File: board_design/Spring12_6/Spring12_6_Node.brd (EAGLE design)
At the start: 100 x 80 mm, 40 parts, among them IC1 L78S05CV, Q1 20MHz, X1 1751248

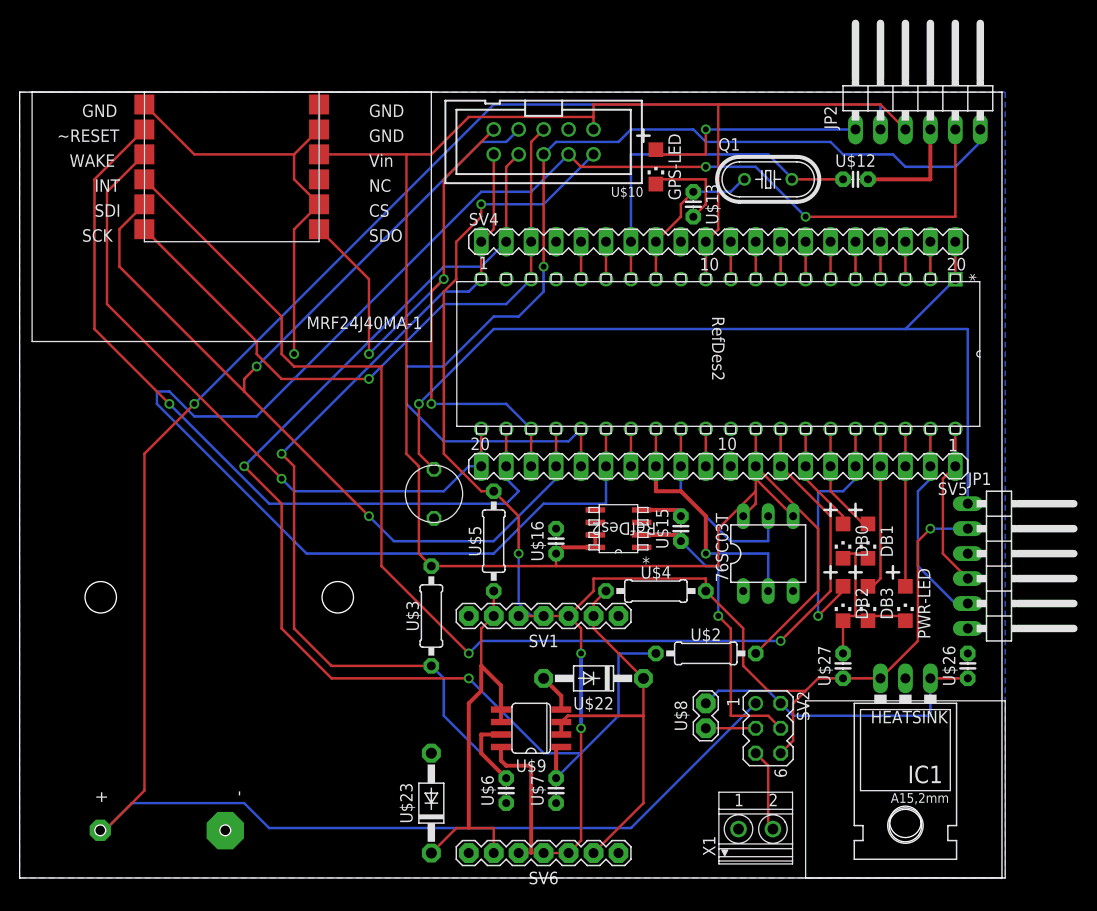
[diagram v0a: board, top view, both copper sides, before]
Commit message: PCB V2
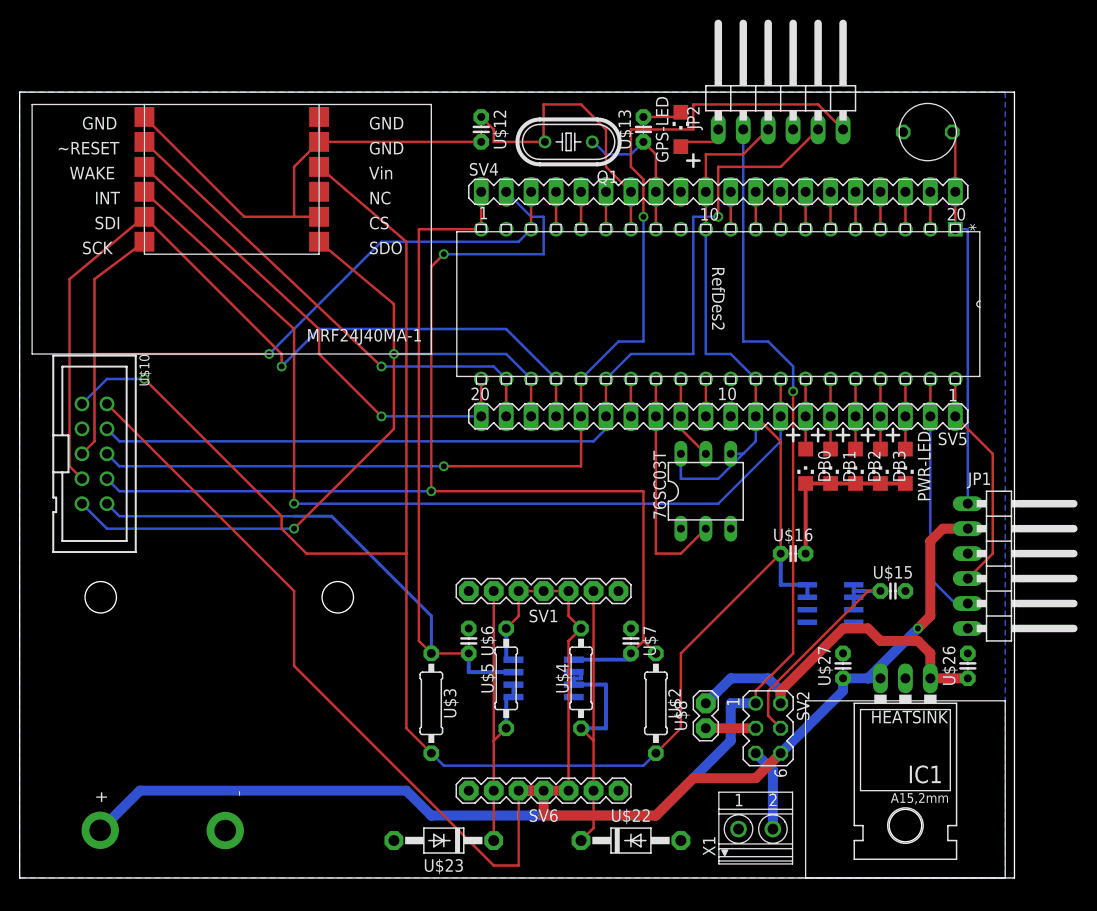
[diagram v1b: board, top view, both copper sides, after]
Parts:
- moved U$25 60.7 mm to (91.4, 74.9), turned to 270 degrees
- moved U$10 55.7 mm to (7.62, 43.2), turned to 270 degrees
- moved U$12 38.4 mm to (47.0, 76.2), turned to 270 degrees
- moved U$16 24.2 mm to (78.7, 33.0), turned to 0 degrees
- moved U$14 22.9 mm to (82.5, 27.9), flipped to the bottom, turned to 0 degrees
- moved U$15 22.5 mm to (88.9, 29.2), turned to 0 degrees
- moved Q1 20.7 mm to (55.9, 74.9), turned to 180 degrees
- moved U$7 17.0 mm to (62.2, 24.1), turned to 270 degrees
- moved U$22 16.9 mm to (62.2, 3.81), turned to 0 degrees
- moved U$6 15.7 mm to (45.7, 24.1), turned to 270 degrees
- moved U$5 14.0 mm to (49.5, 20.3)
- moved DB2 14.0 mm to (85.1, 41.9)
- moved DB3 14.0 mm to (87.6, 41.9)
- moved JP2 14.0 mm to (77.5, 80.0)
- moved PWR-LED 14.0 mm to (90.2, 41.9)
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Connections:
- net N$26: now also U$1.17
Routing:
- net UART-RX: track 167.9 -> 100.2 mm, vias 2 -> 1
- net BATTERY: track 206.7 -> 140.0 mm
- net PIC-RESET: track 95.1 -> 39.8 mm, vias 1 -> 0
- net MRF-RESET: track 80.4 -> 50.3 mm
- net MRF-INT: track 125.2 -> 97.0 mm, vias 2 -> 1
- net VSS: track 96.7 -> 71.8 mm, vias 1 -> 0
- net SPI-MOSI: track 110.9 -> 87.2 mm, vias 2 -> 1
- net 3V3: track 210.4 -> 231.9 mm, vias 0 -> 1
- net DB-LED2: track 26.2 -> 7.62 mm, vias 1 -> 0
- net MRF-WAKE: track 67.7 -> 49.8 mm
- net GPS-LED: track 23.3 -> 5.56 mm, vias 1 -> 0
- net SPI-SCK: track 66.4 -> 78.2 mm
- net I2C-ADDR1: track 19.9 -> 8.67 mm
- net DB-LED3: track 17.5 -> 7.62 mm
- net SDA-BUS: track 41.7 -> 32.4 mm
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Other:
- board size 100 x 80 mm -> 101.3 x 80 mm

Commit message: pcb stuff >_>
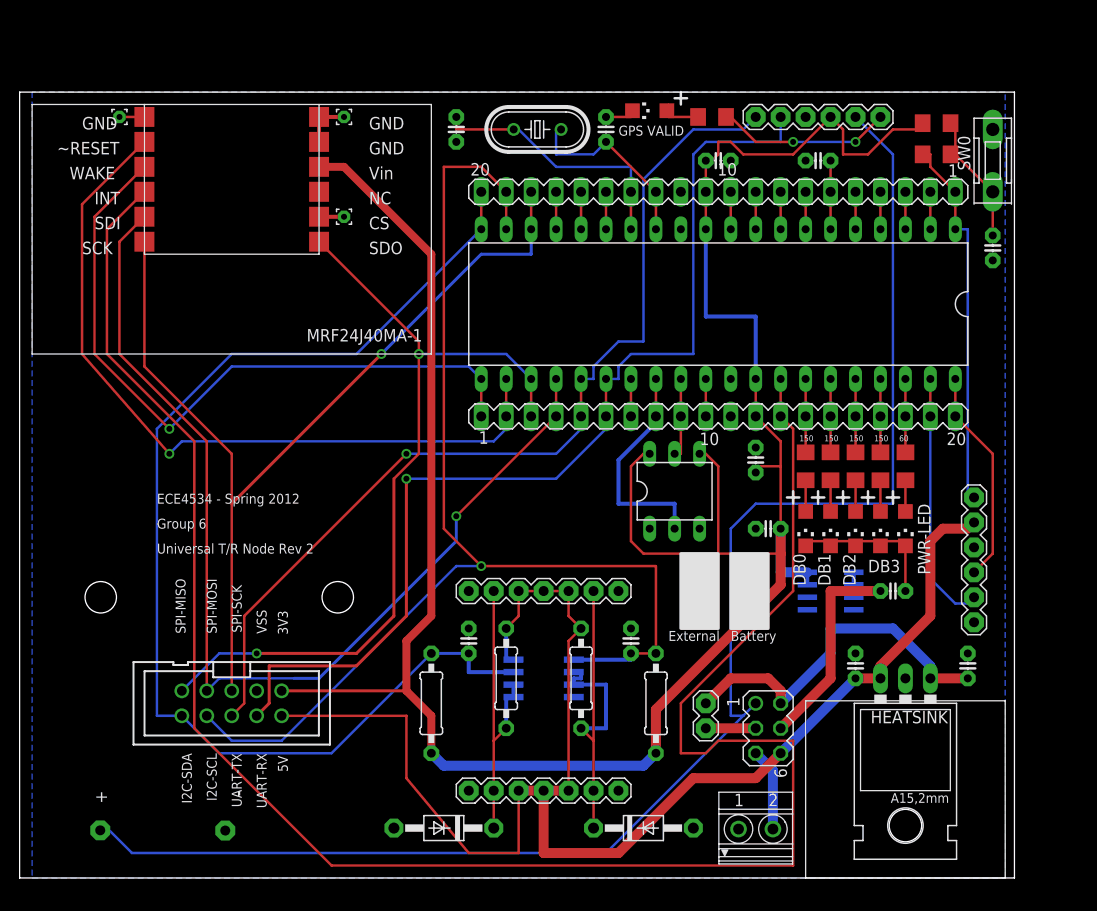
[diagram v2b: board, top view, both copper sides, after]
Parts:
- removed 76SC03T: I2C Select, ic-package:DIL06
- removed JP1: PICKIT, pinhead:1X06/90
- removed JP2: GPSR, pinhead:1X06/90
- removed U$1: PIC18F45J10-X/P, 4534_Node_Board:PDIP40_600MC
- removed U$10: DEBUG, 4534_I2C2:2510-6002
- removed U$12, U$13: 18pF, 4534_I2C2:C2.5-5
- removed U$14: MCP1725-XXXXX/SN, 4534_Node_Board:SOIC8-N_MC
- removed U$16: 10uF, 4534_I2C2:C2.5-5
- removed U$22, U$23: 1N5817P, 4534_I2C2:1N5817
- removed U$25: EVQ-11U05R, 4534_Node_Board:EVQ-11U05R
- removed U$27: 0.1uF, 4534_I2C2:C2.5-5
- added C1, C11, C8, C9: 0.1uF, 4534_I2C2:C2.5-5
- added C10, C7: 10uF, 4534_I2C2:C2.5-5
- added C2, C3: 9pF, 4534_I2C2:C2.5-5
- added D0, D1: 1N5817P, 4534_I2C2:1N5817
- added J2: DEBUG, 4534_I2C2:2510-6002
- added J3: PICKIT, 4534:MA06-1
- added J6: GPSR, 4534:MA06-1
- added PIC0: PIC18F45J10-I/P, 4534:DIL40
- added R10, R11, R8, R9: 150, 4534_I2C2:R1206
- added R4: 10k, 4534_I2C2:R1206
- added R5: 100, 4534_I2C2:R1206
- added R6, R7: 60, 4534_I2C2:R1206
- added REG0: MCP1725-XXXXX/SN, 4534_Node_Board:SOIC8-N_MC
- added SW0: SW-PB-MOM, 4534:SW-MOM-PB
- added SW1: 76SC03T, ic-package:DIL06
- added U$18, U$19, U$20: VIA, 4534_I2C2:VIA
- C4, C5: value 100pF -> 220pF
- moved DB0 6.35 mm to (80.0, 35.6)
- moved DB1 6.35 mm to (82.5, 35.6)
- moved DB2 6.35 mm to (85.1, 35.6)
- moved DB3 6.35 mm to (87.6, 35.6)
- moved PWR-LED 6.35 mm to (90.2, 35.6)
- moved GPS-LED 3.70 mm to (64.1, 78.1), turned to 90 degrees
- moved Q1 3.42 mm to (52.7, 76.2)
- turned J0 to 180 degrees
- turned J1 to 0 degrees
- renumbered IC1 to REG1, SV1 to J4, SV2 to J8, SV4 to J0, SV5 to J1, SV6 to J5, U$11 to RF0, U$15 to C6, U$17 to BATT0, U$2 to R1, U$26 to C0, U$3 to R0, U$4 to R2, U$5 to R3, U$6 to C4, U$7 to C5, U$8 to J9, U$9 to IC0, X1 to J7
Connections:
- new net N$10: DB2.A, R10.2
- new net N$11: DB3.A, R11.2
- new net N$4: GPS-LED.A, R6.2
- new net N$5: PWR-LED.A, R7.2
- new net N$6: C11.1, R4.1, R5.1, SW0.2
- new net N$7: DB0.A, R8.2
- new net N$9: DB1.A, R9.2
- net 3V3: now also C7.1, C8.1, C9.1, J0.11, J1.12, J2.1, J6.4, PIC0.11, PIC0.32, R4.2, REG0.7, REG0.8, SW1.4, SW1.6; no longer 76SC03T.4, 76SC03T.6, J0.10, J1.9, JP2.3, U$1.11, U$1.32, U$10.1, U$14.7, U$14.8, U$16.1
- net 3V3-REG: now also REG0.1, REG0.2, REG0.3; no longer U$14.1, U$14.2, U$14.3
- net 5V: now also C1.1, J2.2, J3.2; no longer JP1.2, U$10.2, U$27.1
- net BATTERY: now also J6.5; no longer JP2.2
- net DB-LED0: now also J1.14, PIC0.34, R8.1; no longer DB0.A, J1.7, U$1.34
- net DB-LED1: now also J1.15, PIC0.35, R9.1; no longer DB1.A, J1.6, U$1.35
- net DB-LED2: now also J1.16, PIC0.36, R10.1; no longer DB2.A, J1.5, U$1.36
- net DB-LED3: now also J1.17, PIC0.37, R11.1; no longer DB3.A, J1.4, U$1.37
- net GPS-LED: now also J6.6, R6.1; no longer GPS-LED.A, JP2.1
- net I2C-ADDR0: now also J1.8, PIC0.28, SW1.2; no longer 76SC03T.2, J1.13, U$1.28
- net I2C-ADDR1: now also J1.9, PIC0.29, SW1.5; no longer 76SC03T.5, J1.12, U$1.29
- net I2C-ADDR2: now also J1.10, PIC0.30; no longer J1.11, U$1.30
- net MRF-INT: now also J1.13, PIC0.33; no longer J1.8, U$1.33
- net MRF-RESET: now also J1.2, PIC0.22; no longer J1.19, U$1.22
- net MRF-WAKE: now also J1.1, PIC0.21; no longer J1.20, U$1.21
- net N$1: now also J0.8, PIC0.8; no longer J0.13, U$1.8
- net N$13: now also J0.2, PIC0.2; no longer J0.19, U$1.2
- net N$14: now also J0.3, PIC0.3; no longer J0.18, U$1.3
- net N$15: now also J0.4, PIC0.4; no longer J0.17, U$1.4
- net N$16: now also J0.5, PIC0.5; no longer J0.16, U$1.5
- net N$17: now also C10.1, J0.6, PIC0.6; no longer J0.15, U$1.6
- net N$18: now also J0.7, PIC0.7; no longer J0.14, U$1.7
- net N$2: now also J0.15, PIC0.15; no longer J0.6, U$1.15
- net N$20: now also J0.9, PIC0.9; no longer J0.12, U$1.9
- net N$21: now also J0.10, PIC0.10; no longer J0.11, U$1.10
- net N$26: now also J0.17, PIC0.17; no longer J0.4, U$1.17
- net N$3: now also J0.16, PIC0.16; no longer J0.5, U$1.16
- net N$8: now also J1.7, PIC0.27; no longer J1.14, U$1.27
- net OSC1: now also C2.1, J0.13, PIC0.13; no longer J0.8, U$1.13, U$13.1
- net OSC2: now also C3.1, J0.14, PIC0.14; no longer J0.7, U$1.14, U$12.1
- net PGC: now also J1.19, J3.5, PIC0.39; no longer J1.2, JP1.5, U$1.39
- net PGD: now also J1.20, J3.4, PIC0.40; no longer J1.1, JP1.4, U$1.40
- net PIC-RESET: now also J0.1, J3.1, PIC0.1, R5.2; no longer J0.20, JP1.1, U$1.1, U$25.P$1
- net PICKIT-AUX: now also J3.6; no longer JP1.6
- net PWR-LED: now also J1.18, PIC0.38, R7.1; no longer J1.3, PWR-LED.A, U$1.38
- net SCL-BUS: now also D1.C; no longer U$22.C
- net SCL-LOCAL: now also J0.19, J2.8, PIC0.19; no longer J0.2, U$10.8
- net SDA-BUS: now also D0.C; no longer U$23.C
- net SDA-LOCAL: now also J0.20, J2.10, PIC0.20; no longer J0.1, U$1.20, U$10.10
- net SPI-MISO: now also J1.3, J2.9, PIC0.23; no longer J1.18, U$1.23, U$10.9
- net SPI-MOSI: now also J1.4, J2.7, PIC0.24; no longer J1.17, U$1.24, U$10.7
- net SPI-SCK: now also J0.18, J2.5, PIC0.18; no longer J0.3, U$1.18, U$10.5
- net UART-RX: now also J1.6, J2.4, J6.2, PIC0.26; no longer J1.15, JP2.5, U$1.26, U$10.4
- net UART-TX: now also J1.5, J2.6, J6.1, PIC0.25; no longer J1.16, JP2.6, U$1.25, U$10.6
- net VSS: now also C1.2, C10.2, C11.2, C2.2, C3.2, C7.2, C8.2, C9.2, D0.A, D1.A, J0.12, J1.11, J2.3, J3.3, J6.3, PIC0.12, PIC0.31, REG0.4, SW0.1, SW1.1, SW1.3, U$18.1, U$19.1, U$20.1; no longer 76SC03T.1, 76SC03T.3, J0.9, J1.10, JP1.3, JP2.4, U$1.12, U$1.31, U$10.3, U$12.2, U$13.2, U$14.4, U$16.2, U$22.A, U$23.A, U$25.P$2, U$27.2
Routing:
- net MRF-INT: track 97.0 -> 194.6 mm, vias 1 -> 0
- net VSS: track 71.8 -> 30.5 mm
- net 5V: track 182.6 -> 149.5 mm, vias 1 -> 0
- net MRF-RESET: track 50.3 -> 78.1 mm
- net 3V3: track 231.9 -> 256.1 mm, vias 1 -> 0
- net MRF-WAKE: track 49.8 -> 70.6 mm
- net SPI-SCK: track 78.2 -> 96.8 mm
- net SPI-MOSI: track 87.2 -> 105.4 mm
- net UART-TX: track 112.9 -> 97.2 mm, vias 2 -> 1
- net N$6: track 0.00 -> 13.7 mm
- net BATTERY: track 140.0 -> 153.0 mm, vias 1 -> 0
- net SDA-LOCAL: track 105.7 -> 118.4 mm
- net GPS-LED: track 5.56 -> 17.8 mm, vias 0 -> 2
- net SPI-MISO: track 78.5 -> 84.4 mm
- net UART-RX: track 100.2 -> 106.1 mm
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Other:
- board text added: "150"
- board text added: "3V3"
- board text added: "5V"
- board text added: "60"
- board text added: "Battery"
- board text added: "ECE4534 - Spring 2012"
- board text added: "External"
- board text added: "GPS VALID"
- board text added: "Group 6"
- board text added: "I2C-SCL"
- board text added: "I2C-SDA"
- board text added: "MCP1725-3302E/SN"
- board text added: "SPI-MISO"
- board text added: "SPI-MOSI"
- board text added: "SPI-SCK"
- board text added: "UART-RX"
- board text added: "UART-TX"
- board text added: "Universal T/R Node Rev 2"
- board text added: "VSS"
